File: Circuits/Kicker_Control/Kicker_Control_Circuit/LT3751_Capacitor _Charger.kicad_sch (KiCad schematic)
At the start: 7 parts, among them Q2 NMOS, U4 VS-5EWH06FN-M3

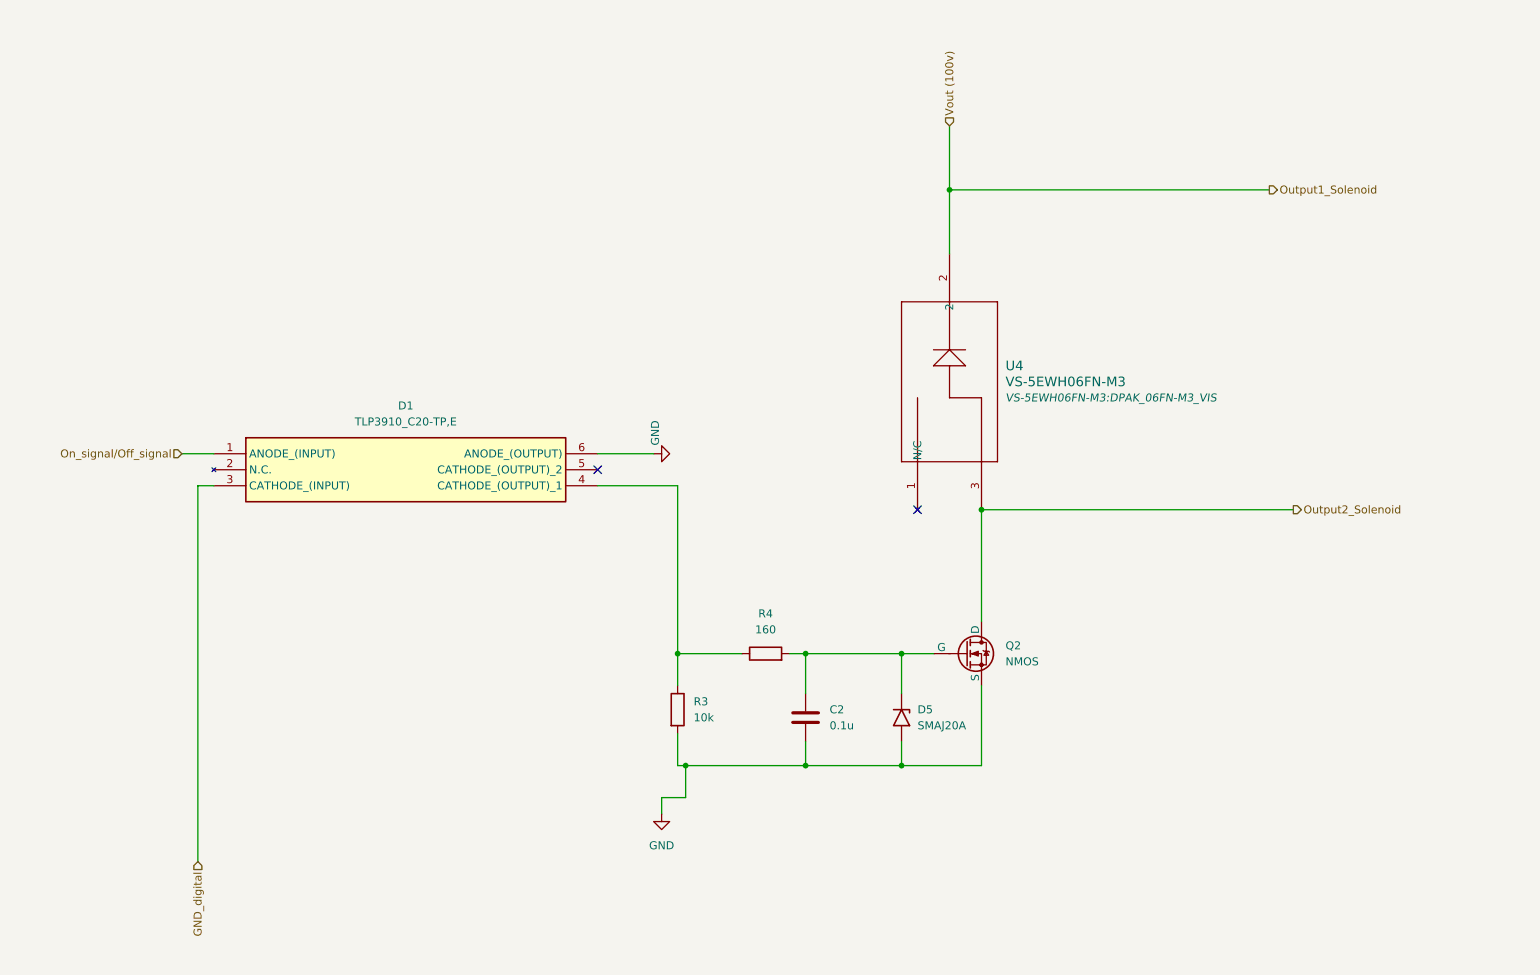
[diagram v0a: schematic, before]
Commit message: Changes in the circuit
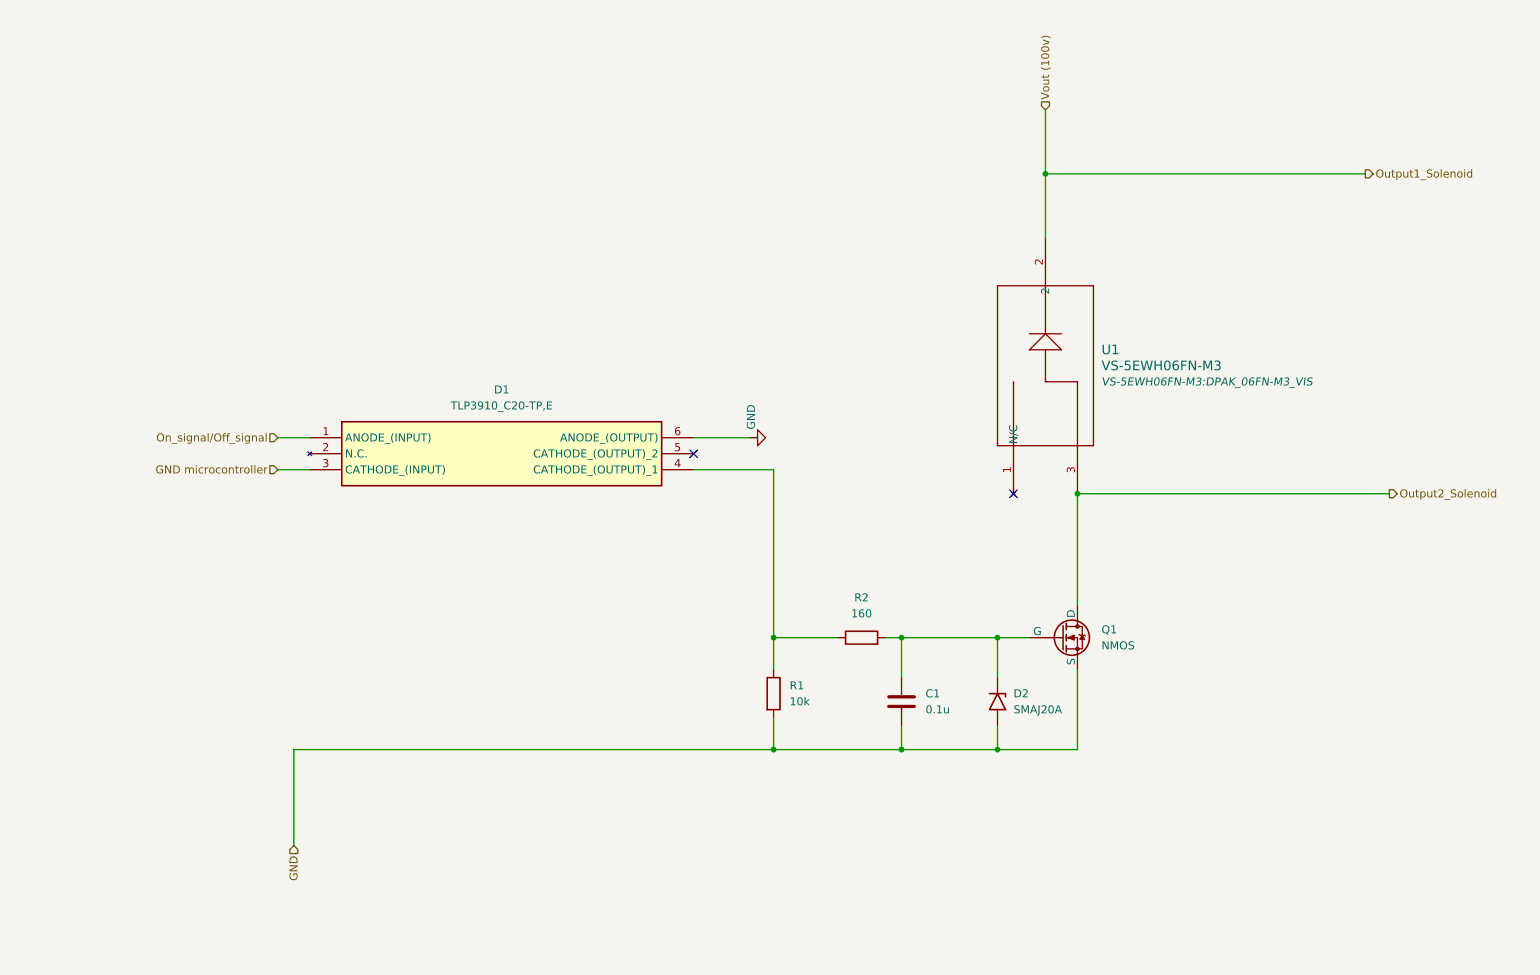
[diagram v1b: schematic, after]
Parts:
- removed C2: 0.1u, symbol Device:C
- removed D5: SMAJ20A, SMAJ20A:DIOM4325X250N, symbol Diode:SMAJ20A
- removed Q2: NMOS, symbol Simulation_SPICE:NMOS
- removed R3: 10k, symbol Device:R
- removed R4: 160, symbol Device:R
- removed U4: VS-5EWH06FN-M3, VS-5EWH06FN-M3:DPAK_06FN-M3_VIS, symbol VS-5EWH06FN-M3:VS-5EWH06FN-M3
- added C1: 0.1u, symbol Device:C
- added D2: SMAJ20A, SMAJ20A:DIOM4325X250N, symbol Diode:SMAJ20A
- added Q1: NMOS, symbol Simulation_SPICE:NMOS
- added R1: 10k, symbol Device:R
- added R2: 160, symbol Device:R
- added U1: VS-5EWH06FN-M3, VS-5EWH06FN-M3:DPAK_06FN-M3_VIS, symbol VS-5EWH06FN-M3:VS-5EWH06FN-M3
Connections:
- net GND: now also C1.2, D2.2 (A2), Q1.3 (S), R1.2
- net Output1_Solenoid: now also U1.2
- net Output2_Solenoid: now also Q1.1 (D), U1.3
- net at D1.4 (CATHODE_(OUTPUT)_1): now also R1.1, R2.1
- net GND_digital renamed GND microcontroller
- new net: C1.1, D2.1 (A1), Q1.2 (G), R2.2
